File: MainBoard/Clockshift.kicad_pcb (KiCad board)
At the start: 4 copper layers, 10.4 x 18 mm, 7 parts, among them J1 Conn_01x04, SW1 CS-4-13, U1 LTC6905

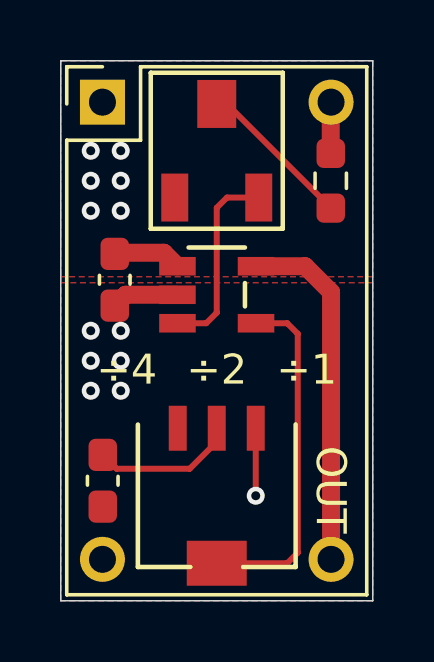
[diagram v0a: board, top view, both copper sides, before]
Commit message: Design rules and gerber files
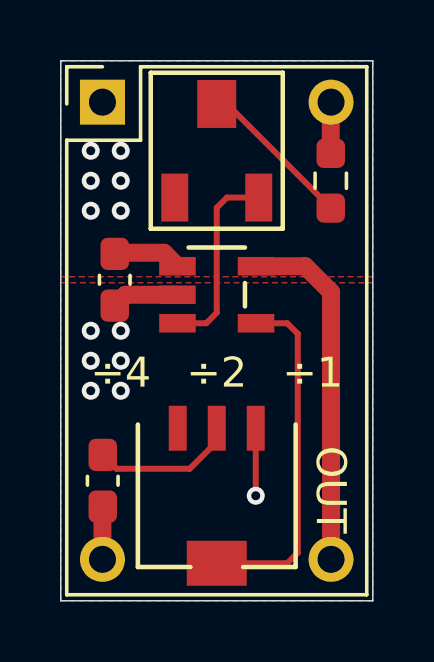
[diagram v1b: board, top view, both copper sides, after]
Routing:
- net GND: track 2.25 -> 4.02 mm
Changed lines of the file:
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@@
 			(plot_on_all_layers_selection 0x0000000_00000000)
 			(disableapertmacros no)
-			(usegerberextensions no)
+			(usegerberextensions yes)
 			(usegerberattributes yes)
 			(usegerberadvancedattributes yes)
-			(creategerberjobfile yes)
+			(creategerberjobfile no)
 			(dashed_line_dash_ratio 12.000000)
 			(dashed_line_gap_ratio 3.000000)
@@
 			(psa4output no)
 			(plotreference yes)
-			(plotvalue yes)
+			(plotvalue no)
 			(plotfptext yes)
 			(plotinvisibletext no)
 			(sketchpadsonfab no)
-			(subtractmaskfromsilk no)
+			(subtractmaskfromsilk yes)
 			(outputformat 1)
 			(mirror no)
-			(drillshape 1)
+			(drillshape 0)
 			(scaleselection 1)
 			(outputdirectory "")
@@
 	)
 	(gr_text "÷4"
-		(at 102.2 110.3 0)
+		(at 102 110.4 0)
 		(layer "F.SilkS")
 		(effects
@@
 	)
 	(gr_text "÷1"
-		(at 108.2 110.3 0)
+		(at 108.4 110.4 0)
 		(layer "F.SilkS")
 		(effects
@@
 	)
 	(gr_text "÷2"
-		(at 105.2 110.3 0)
+		(at 105.2 110.4 0)
 		(layer "F.SilkS")
 		(effects
@@
 	)
 	(segment
+		(start 101.39 114.8725)
+		(end 101.4 114.8625)
+		(width 0.2)
+		(layer "F.Cu")
+		(net 2)
+	)
+	(segment
 		(start 101.4 116.61)
 		(end 101.39 116.62)
@@
 		(width 0.6)
 		(layer "F.Cu")
+		(net 2)
+	)
+	(segment
+		(start 101.39 116.62)
+		(end 101.39 114.8725)
+		(width 0.6)
+		(layer "F.Cu")
